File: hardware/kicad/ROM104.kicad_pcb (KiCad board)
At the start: 2 copper layers, 100 x 85 mm, 58 parts, among them J1 Screw_Terminal_01x03, J2 Screw_Terminal_01x03, J3 CAN, J4 Screw_Terminal_01x03, J5 Screw_Terminal_01x03, J6 Screw_Terminal_01x03, J7 Screw_Terminal_01x03, K1 PE014F05, K2 PE014F05, K3 PE014F05, K4 PE014F05, K5 PE014F05, K6 PE014F05, SW1 INSTANCE, SW2 BUS, SW3 PRG, U1 L293D, U2 MCP2551-I-P, U3 TMR_2411, U4 L293D, U5 L293D, U6 74HC595, U7 Teensy_3.2, U8 MAX6816

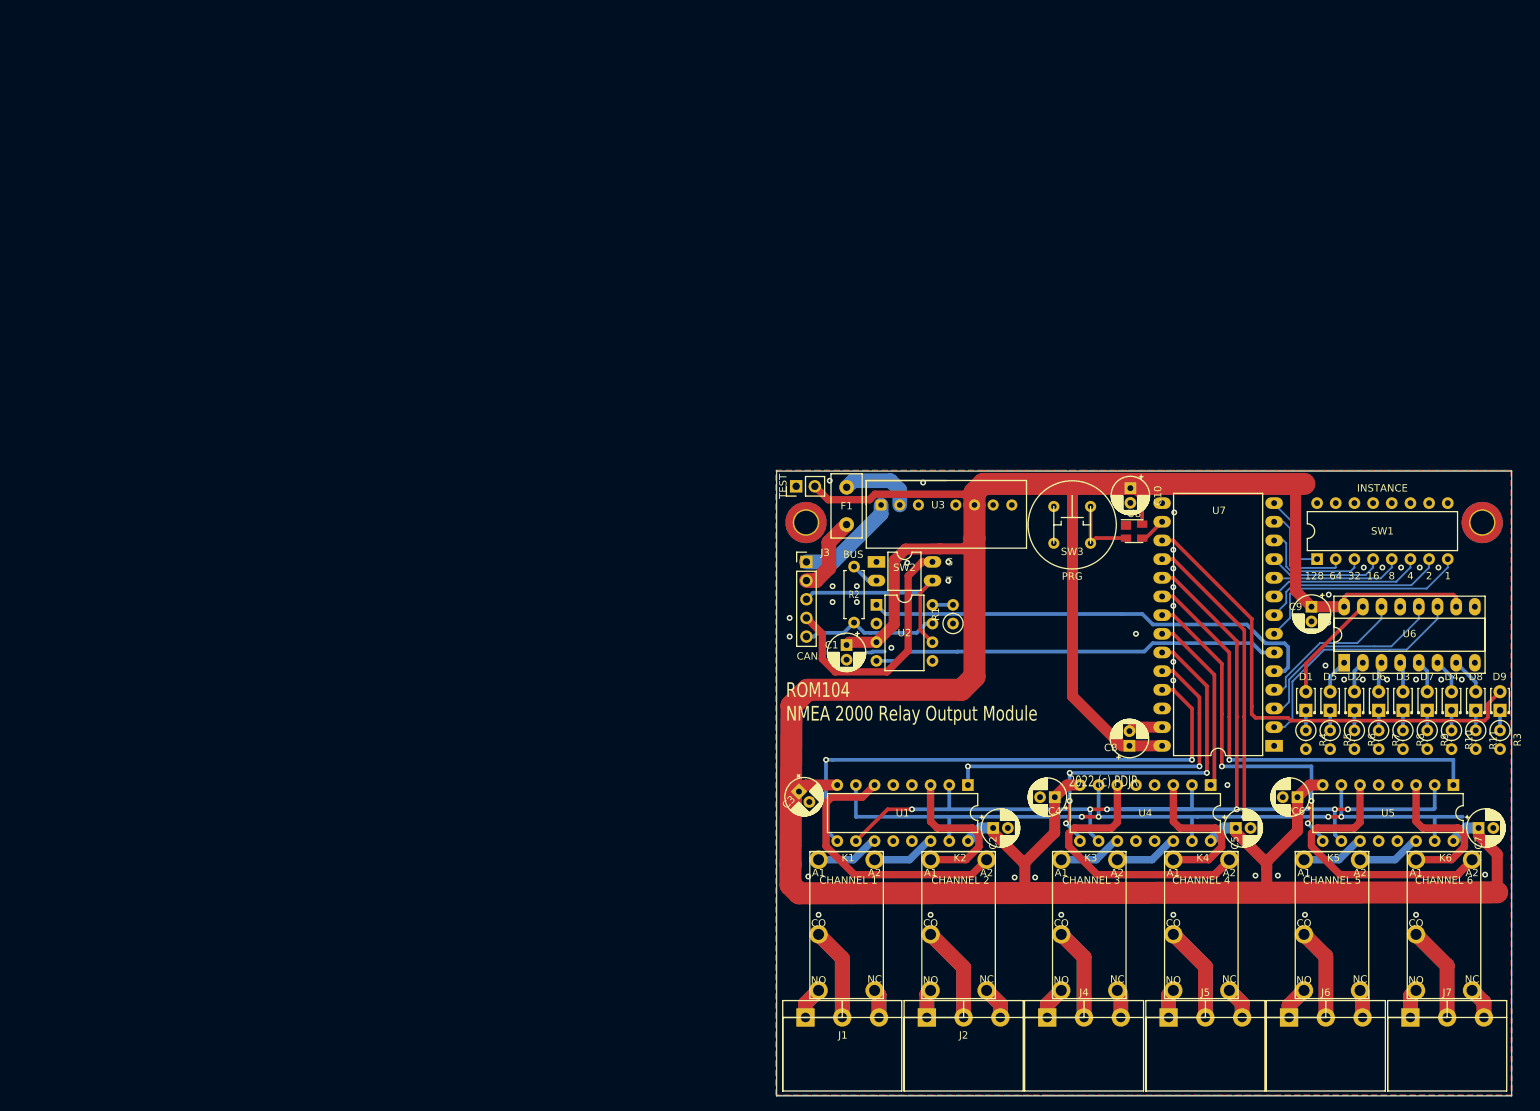
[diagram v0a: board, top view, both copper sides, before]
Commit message: Tweak
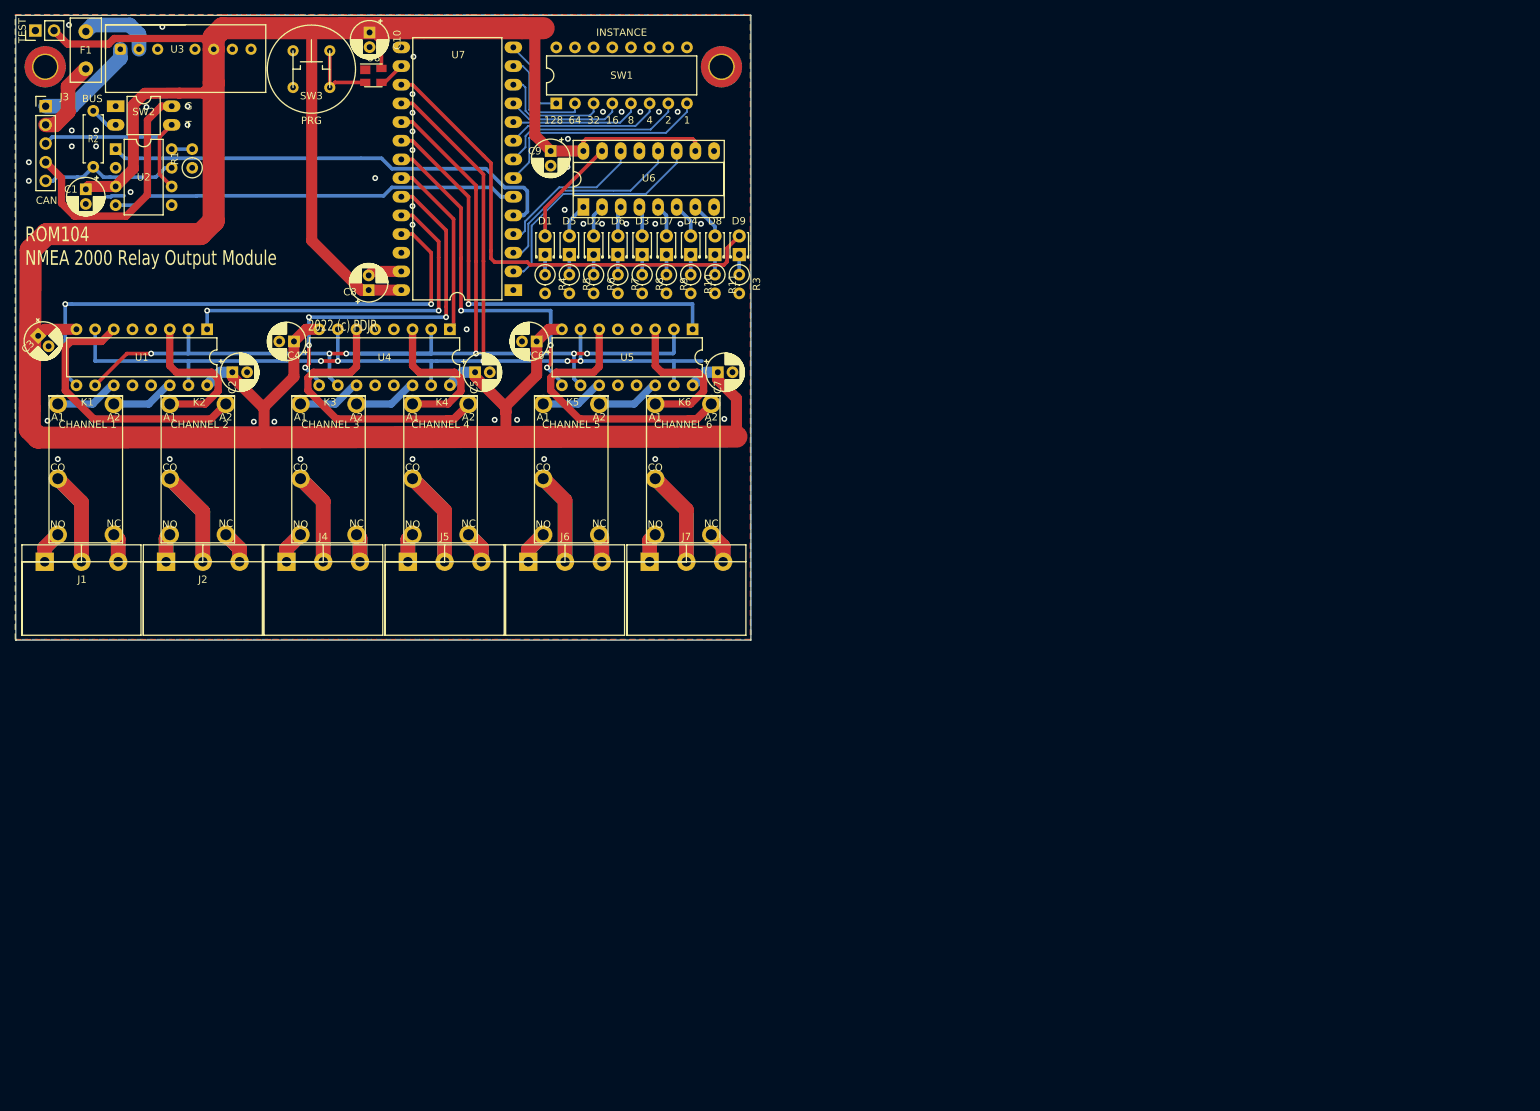
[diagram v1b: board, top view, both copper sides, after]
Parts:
- removed the REF** at (127.5, 89.0)
- removed the REF** at (219.5, 89.0)
- added REF**: MountingHole_3.2mm_M3_DIN965_Pad_TopBottom, MountingHole:MountingHole_3.2mm_M3_DIN965_Pad_TopBottom, F.Cu at (24.0, 27.0)
- added REF**: MountingHole_3.2mm_M3_DIN965_Pad_TopBottom, MountingHole:MountingHole_3.2mm_M3_DIN965_Pad_TopBottom, F.Cu at (116.0, 27.0)
- moved C1 120.6 mm to (29.5, 43.7)
- moved C5 120.6 mm to (82.5, 68.6)
- moved D5 120.6 mm to (95.3, 52.6)
- moved D7 120.6 mm to (108.5, 52.6)
- moved F1 120.6 mm to (29.5, 27.3)
- moved J5 120.6 mm to (73.3, 94.3)
- moved J7 120.6 mm to (106.2, 94.3)
- moved K6 120.6 mm to (107.0, 90.7)
- moved R5 120.6 mm to (95.3, 55.3)
- moved R9 120.6 mm to (108.5, 55.3)
- moved U4 120.6 mm to (79.0, 62.7)
- moved U6 120.6 mm to (97.2, 46.1)
- moved C2 120.6 mm to (49.5, 68.6)
- moved C3 120.6 mm to (23.0, 63.6)
- moved C4 120.6 mm to (57.8, 64.4)
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
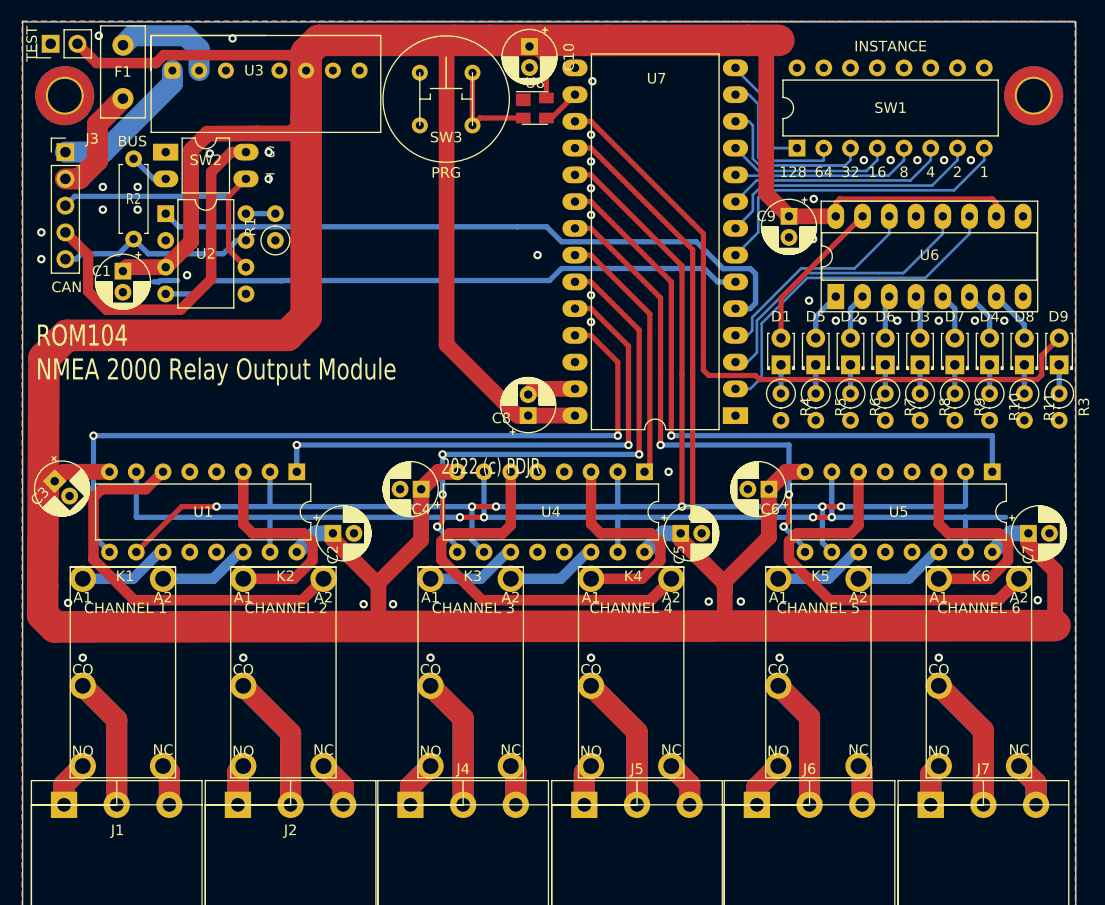
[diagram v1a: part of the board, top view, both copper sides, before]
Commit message: Tweak
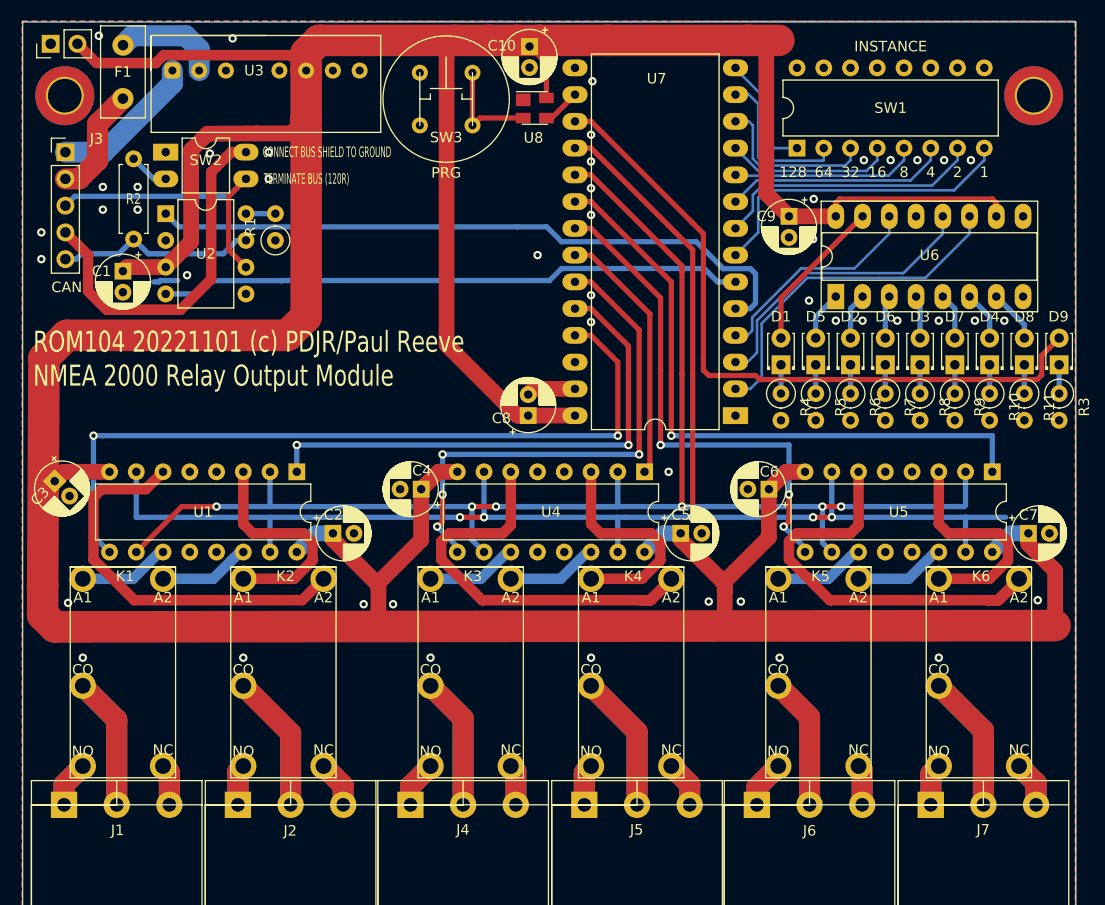
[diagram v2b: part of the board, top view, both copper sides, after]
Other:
- board text added: "CONNECT BUS SHIELD TO GROUND"
- board text added: "ROM104 20221101 (c) PDJR/Paul Reeve NMEA 2000 Relay Output Module"
- board text added: "TERMINATE BUS (120R)"
- board text removed: "2022 (c) PDJR"
- board text removed: "CHANNEL 1"
- board text removed: "CHANNEL 2"
- board text removed: "CHANNEL 3"
- board text removed: "CHANNEL 4"
- board text removed: "CHANNEL 5"
- board text removed: "CHANNEL 6"
- board text removed: "G"
- board text removed: "ROM104 NMEA 2000 Relay Output Module"
- board text removed: "T"
